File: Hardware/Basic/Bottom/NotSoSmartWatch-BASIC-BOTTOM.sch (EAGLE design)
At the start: 32 parts, among them U1 AD5242-SO16

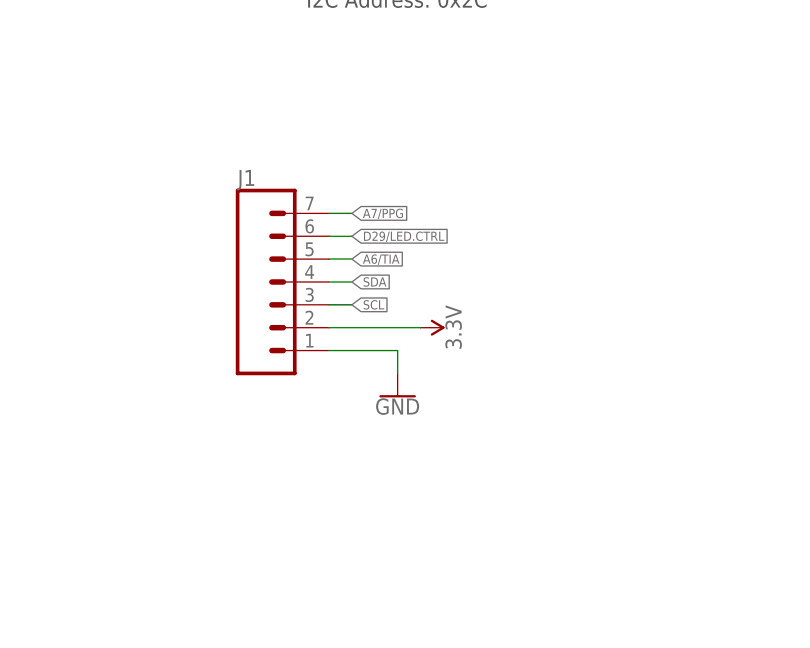
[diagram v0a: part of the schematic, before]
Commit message: still working through Take 003
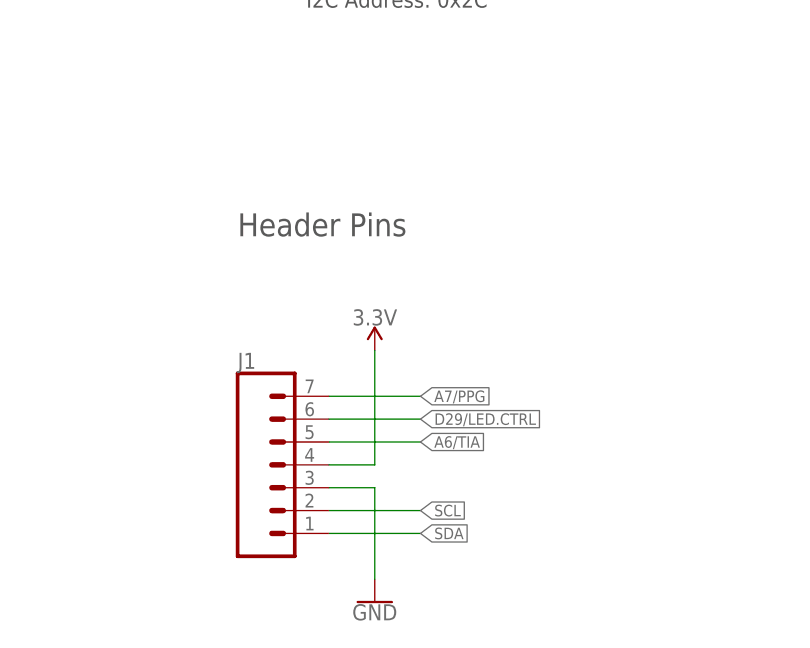
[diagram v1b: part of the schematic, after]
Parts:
- J1: device LinnesLab-Connectors:CONN_07 -> LinnesLab-Connectors:CONN_07-1.27MM
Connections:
- net 3.3V: now also J1.4; no longer J1.2
- net GND: now also J1.3; no longer J1.1
- net SCL: now also J1.2; no longer J1.3
- net SDA: now also J1.1; no longer J1.4
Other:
- note added: "Header Pins"
- moved on the sheet: J1
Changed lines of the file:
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@@
 <part name="GND2" library="LinnesLab-Symbols" deviceset="GND" device=""/>
 <part name="SUPPLY3" library="LinnesLab-Symbols" deviceset="3.3V" device=""/>
-<part name="J1" library="LinnesLab-Connectors" deviceset="CONN_07" device=""/>
+<part name="J1" library="LinnesLab-Connectors" deviceset="CONN_07" device="-1.27MM"/>
+<part name="SUPPLY1" library="LinnesLab-Symbols" deviceset="3.3V" device=""/>
 <part name="GND3" library="LinnesLab-Symbols" deviceset="GND" device=""/>
-<part name="SUPPLY1" library="LinnesLab-Symbols" deviceset="3.3V" device=""/>
 </parts>
 <sheets>
@@
 <text x="144.78" y="35.56" size="1.778" layer="97" ratio="15">I2C Address: 0x2C</text>
 <text x="210.82" y="38.1" size="1.778" layer="97" ratio="15">I2C Address: 0x2D</text>
+<text x="137.16" y="10.16" size="2.54" layer="97" font="vector" ratio="15">Header Pins</text>
 </plain>
 <instances>
@@
 <attribute name="VALUE" x="27.94" y="25.654" size="1.778" layer="96" align="bottom-center"/>
 </instance>
-<instance part="J1" gate="G$1" x="142.24" y="2.54" smashed="yes">
-<attribute name="VALUE" x="137.16" y="-7.366" size="1.778" layer="96" font="vector"/>
-<attribute name="NAME" x="137.16" y="15.748" size="1.778" layer="95" font="vector"/>
-</instance>
-<instance part="GND3" gate="G$1" x="154.94" y="-7.62" smashed="yes">
-<attribute name="VALUE" x="154.94" y="-7.874" size="1.778" layer="96" align="top-center"/>
-</instance>
-<instance part="SUPPLY1" gate="G$1" x="157.48" y="0" smashed="yes" rot="R270">
-<attribute name="VALUE" x="160.274" y="0" size="1.778" layer="96" rot="R270" align="bottom-center"/>
+<instance part="J1" gate="G$1" x="142.24" y="-17.78" smashed="yes">
+<attribute name="VALUE" x="137.16" y="-27.686" size="1.778" layer="96" font="vector"/>
+<attribute name="NAME" x="137.16" y="-4.572" size="1.778" layer="95" font="vector"/>
+</instance>
+<instance part="SUPPLY1" gate="G$1" x="152.4" y="-2.54" smashed="yes">
+<attribute name="VALUE" x="152.4" y="0.254" size="1.778" layer="96" align="bottom-center"/>
+</instance>
+<instance part="GND3" gate="G$1" x="152.4" y="-30.48" smashed="yes">
+<attribute name="VALUE" x="152.4" y="-30.734" size="1.778" layer="96" align="top-center"/>
 </instance>
 </instances>
@@
 </segment>
 <segment>
-<pinref part="J1" gate="G$1" pin="1"/>
-<wire x1="147.32" y1="-2.54" x2="154.94" y2="-2.54" width="0.1524" layer="91"/>
+<pinref part="J1" gate="G$1" pin="3"/>
+<wire x1="147.32" y1="-17.78" x2="152.4" y2="-17.78" width="0.1524" layer="91"/>
 <pinref part="GND3" gate="G$1" pin="GND"/>
-<wire x1="154.94" y1="-2.54" x2="154.94" y2="-5.08" width="0.1524" layer="91"/>
+<wire x1="152.4" y1="-17.78" x2="152.4" y2="-27.94" width="0.1524" layer="91"/>
 </segment>
 </net>
@@
 </segment>
 <segment>
-<pinref part="J1" gate="G$1" pin="2"/>
+<pinref part="J1" gate="G$1" pin="4"/>
+<wire x1="147.32" y1="-15.24" x2="152.4" y2="-15.24" width="0.1524" layer="91"/>
 <pinref part="SUPPLY1" gate="G$1" pin="3.3V"/>
-<wire x1="157.48" y1="0" x2="147.32" y2="0" width="0.1524" layer="91"/>
+<wire x1="152.4" y1="-15.24" x2="152.4" y2="-2.54" width="0.1524" layer="91"/>
 </segment>
 </net>
@@
 </segment>
 <segment>
-<pinref part="J1" gate="G$1" pin="4"/>
-<wire x1="147.32" y1="5.08" x2="149.86" y2="5.08" width="0.1524" layer="91"/>
-<label x="149.86" y="5.08" size="1.016" layer="95" xref="yes"/>
+<pinref part="J1" gate="G$1" pin="1"/>
+<wire x1="147.32" y1="-22.86" x2="157.48" y2="-22.86" width="0.1524" layer="91"/>
+<label x="157.48" y="-22.86" size="1.27" layer="95" xref="yes"/>
 </segment>
 </net>
@@
 </segment>
 <segment>
-<pinref part="J1" gate="G$1" pin="3"/>
-<wire x1="147.32" y1="2.54" x2="149.86" y2="2.54" width="0.1524" layer="91"/>
-<label x="149.86" y="2.54" size="1.016" layer="95" xref="yes"/>
+<pinref part="J1" gate="G$1" pin="2"/>
+<wire x1="147.32" y1="-20.32" x2="157.48" y2="-20.32" width="0.1524" layer="91"/>
+<label x="157.48" y="-20.32" size="1.27" layer="95" xref="yes"/>
 </segment>
 </net>
@@
 <segment>
 <pinref part="J1" gate="G$1" pin="5"/>
-<wire x1="147.32" y1="7.62" x2="149.86" y2="7.62" width="0.1524" layer="91"/>
-<label x="149.86" y="7.62" size="1.016" layer="95" xref="yes"/>
+<wire x1="147.32" y1="-12.7" x2="157.48" y2="-12.7" width="0.1524" layer="91"/>
+<label x="157.48" y="-12.7" size="1.27" layer="95" xref="yes"/>
 </segment>
 </net>
@@
 <segment>
 <pinref part="J1" gate="G$1" pin="6"/>
-<wire x1="147.32" y1="10.16" x2="149.86" y2="10.16" width="0.1524" layer="91"/>
-<label x="149.86" y="10.16" size="1.016" layer="95" xref="yes"/>
+<wire x1="147.32" y1="-10.16" x2="157.48" y2="-10.16" width="0.1524" layer="91"/>
+<label x="157.48" y="-10.16" size="1.27" layer="95" xref="yes"/>
 </segment>
 </net>
@@
 <segment>
 <pinref part="J1" gate="G$1" pin="7"/>
-<wire x1="147.32" y1="12.7" x2="149.86" y2="12.7" width="0.1524" layer="91"/>
-<label x="149.86" y="12.7" size="1.016" layer="95" xref="yes"/>
-</segment>
-</net>
+<wire x1="147.32" y1="-7.62" x2="157.48" y2="-7.62" width="0.1524" layer="91"/>
+<label x="157.48" y="-7.62" size="1.27" layer="95" xref="yes"/>
+</segment>
+</net>
